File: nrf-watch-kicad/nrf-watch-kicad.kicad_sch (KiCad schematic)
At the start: 73 parts, among them IC1 TLV840MAPL36DBVRQ1, IC2 XC9265C181MR-G, IC3 TPS61023DRLT, IC4 MAX30101EFD+T, J1 Conn_ARM_JTAG_SWD_10, M1 Vibrator DC Motor, Q1 DMP2045U-7, Q2 S8050, U1 MAX1811ESA+, U2 DMC2400UV-7, U3 LIS2DS12TR, U4 MX25R6435FZNIL0, U5 u-blox ANNA-B402, U6 DRV2603RUNT, U7 XC9265A331MR-G, U8 TXB0104QRUTRQ1, U9 GC9A01

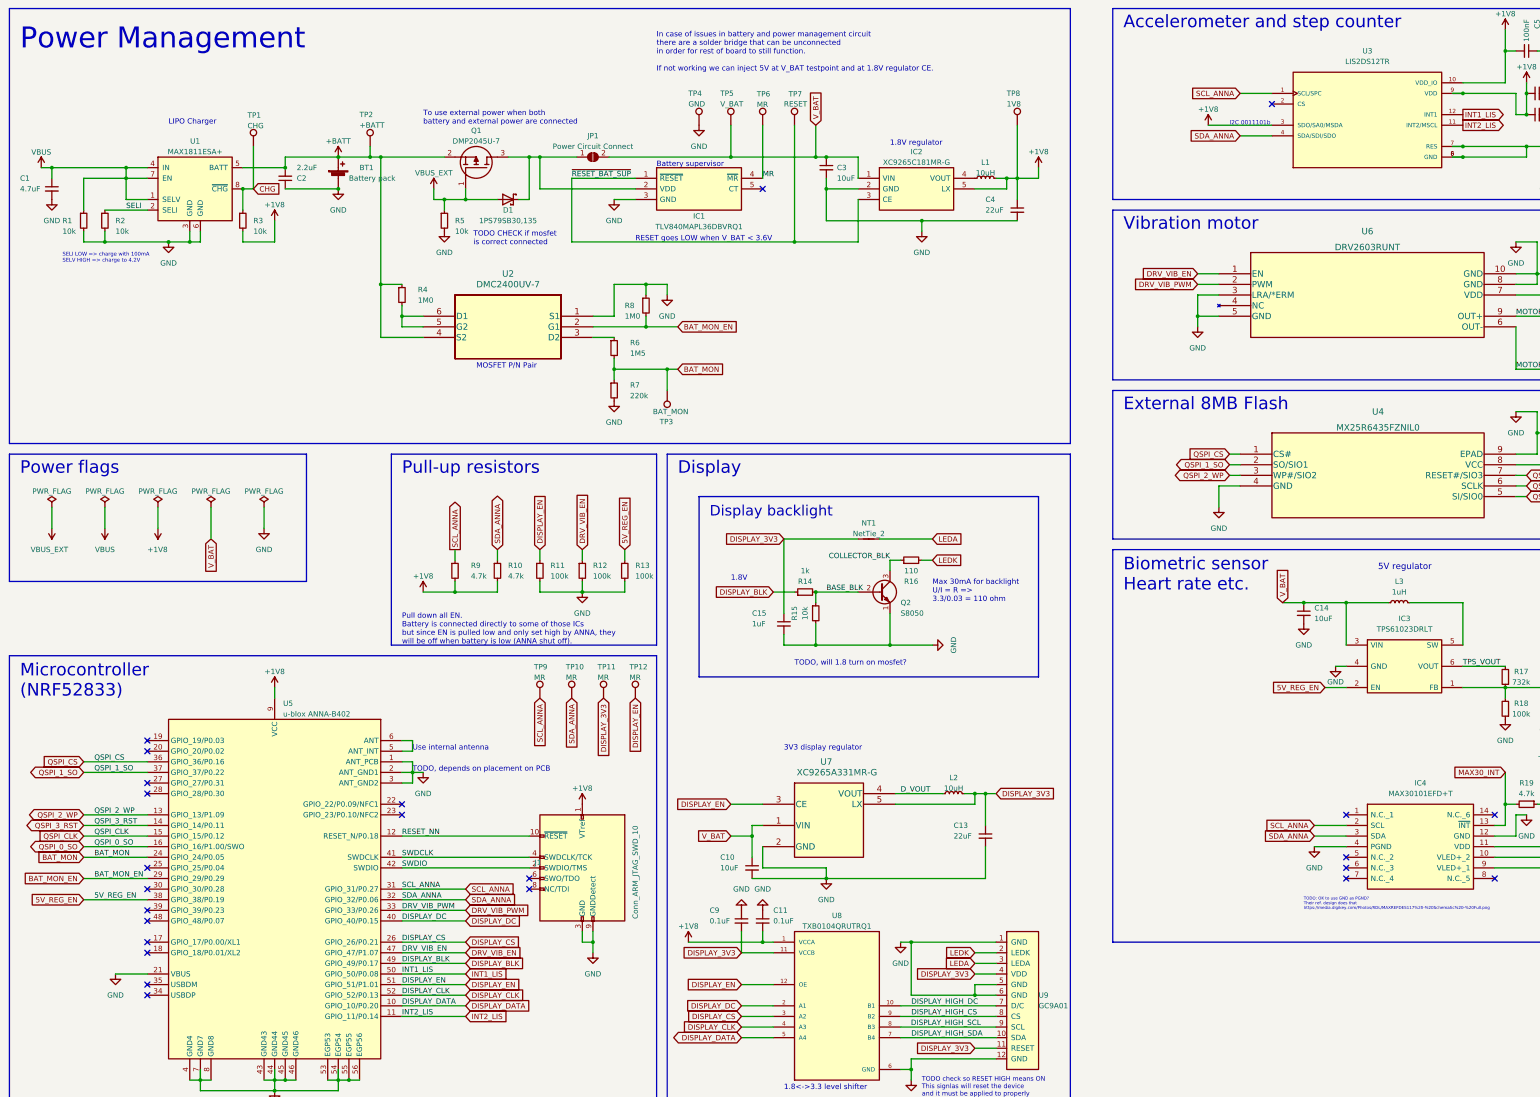
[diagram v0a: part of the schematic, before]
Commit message: Started with routing.
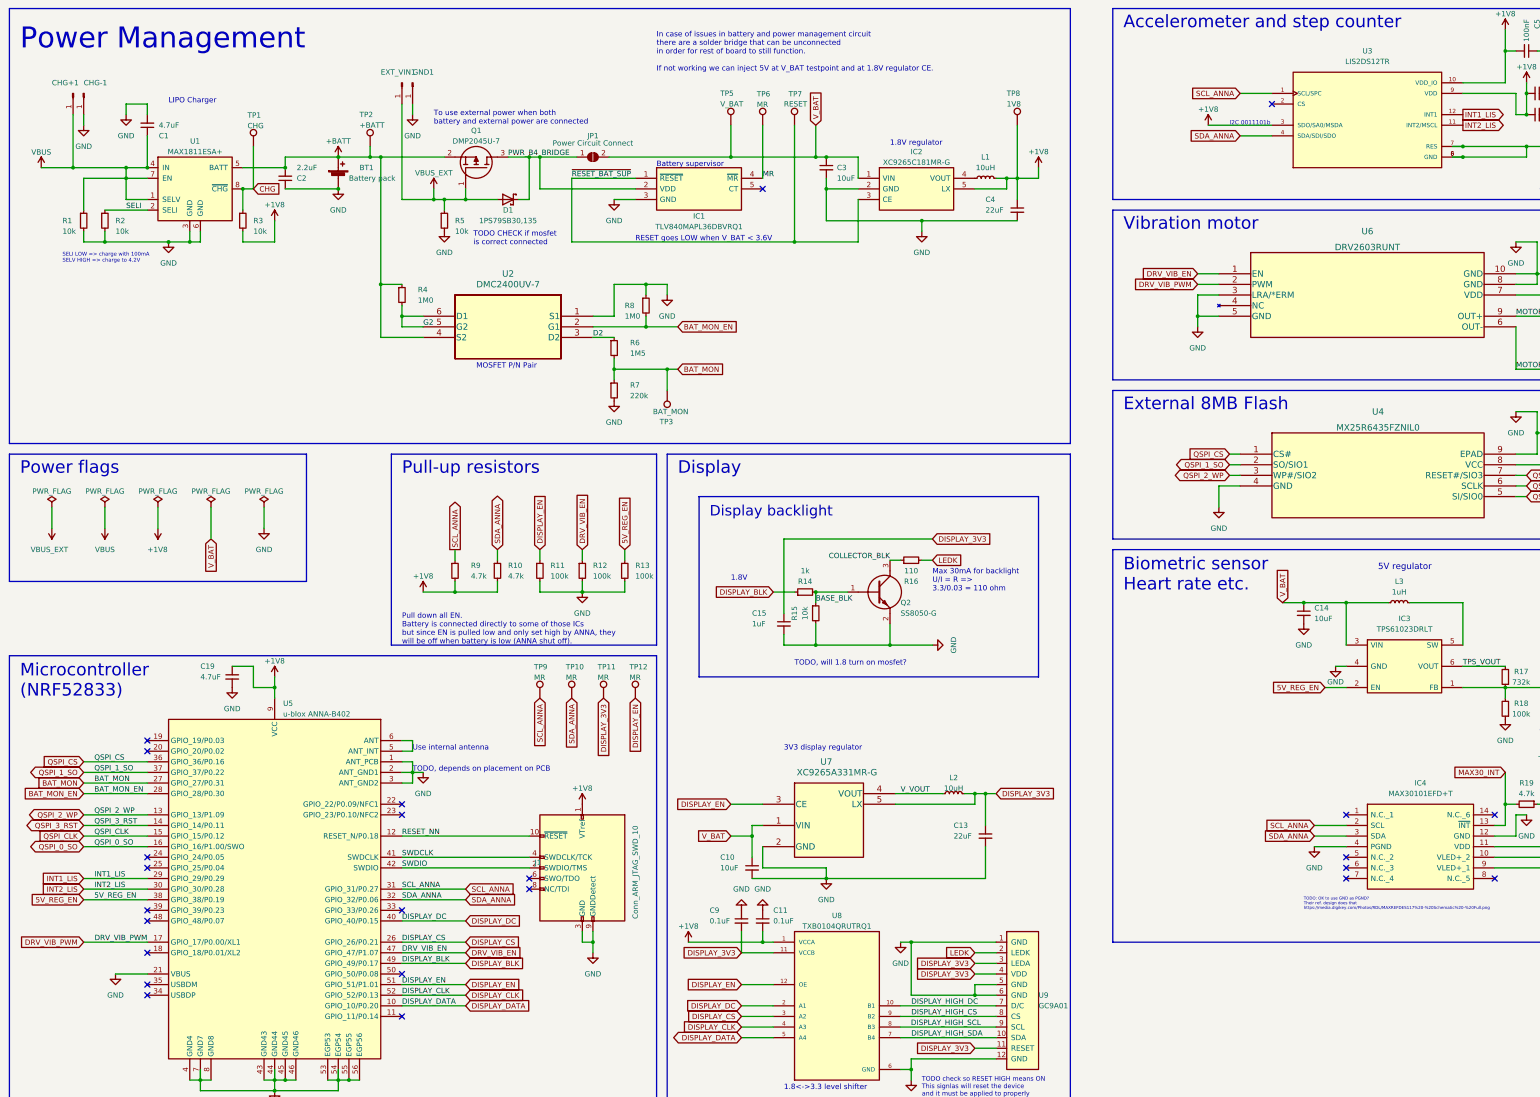
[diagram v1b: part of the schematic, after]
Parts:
- removed NT1: NetTie_2, symbol Device:NetTie_2
- removed Q2: S8050, symbol Transistor_BJT:S8050
- removed TP4: GND, TestPoint:TestPoint_Pad_D2.0mm, symbol Connector:TestPoint
- added C19: 4.7uF, Capacitor_SMD:C_0603_1608Metric_Pad1.08x0.95mm_HandSolder, symbol Device:C_Small
- added CHG+1, EXT_VIN1: Conn_01x01_Male, TestPoint:TestPoint_Pad_D1.5mm, symbol Connector:Conn_01x01_Male
- added CHG-1, GND1: Conn_01x01_Male, TestPoint:TestPoint_Pad_1.5x1.5mm, symbol Connector:Conn_01x01_Male
- added Q2: SS8050-G, SamacSys_Parts:SOT95P240X115-3N, symbol SamacSys_Parts:SS8050-G
- BT1: footprint (none) -> Connector_Wire:SolderWire-0.1sqmm_1x02_P3.6mm_D0.4mm_OD1mm
- L1, L2, L3: footprint (none) -> Inductor_SMD:L_0603_1608Metric_Pad1.05x0.95mm_HandSolder
- M1: footprint (none) -> user_library:TestPoint_2Pads_Pitch2.54mm_Drill0.8mm
- TP5, TP8: footprint TestPoint:TestPoint_Pad_D2.0mm -> TestPoint:TestPoint_Pad_D1.0mm
- U5: footprint user_library:ANNA-B402 -> user_library:ANNA-B402_altium_import
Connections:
- net LEDA is gone; now on net DISPLAY_3V3: U9.3 (LEDA)
- net +1V8: now also C19.1
- net BASE_BLK: now also Q2.1
- net BAT_MON: now also U5.27 (GPIO_27/P0.31); no longer U5.24 (GPIO_24/P0.05)
- net BAT_MON_EN: now also U5.28 (GPIO_28/P0.30); no longer U5.29 (GPIO_29/P0.29)
- net COLLECTOR_BLK: now also Q2.3
- net DRV_VIB_PWM: now also U5.17 (GPIO_17/P0.00/XL1); no longer U5.33 (GPIO_33/P0.26)
- net GND: now also C19.2, CHG-1.1 (Pin_1), GND1.1 (Pin_1), Q2.2
- net INT1_LIS: now also U5.29 (GPIO_29/P0.29); no longer U5.50 (GPIO_50/P0.08)
- net INT2_LIS: now also U5.30 (GPIO_30/P0.28); no longer U5.11 (GPIO_11/P0.14)
- net VBUS: now also CHG+1.1 (Pin_1)
- net VDDA: now also EXT_VIN1.1 (Pin_1)
- net PWR_B4_BRIDGE: now reaches D1.1, IC1.2 (VDD), JP1.1 (A), Q1.3
- net D2: now reaches R6.1, U2.3 (D2)
- net G2: now reaches R4.2, U2.5 (G2), U2.6 (D1)
- net D_VOUT renamed V_VOUT
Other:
- moved on the sheet: C1
